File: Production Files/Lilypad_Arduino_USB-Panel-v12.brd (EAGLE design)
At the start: 125.7 x 125.7 mm, 187 parts, among them U1 MCP73831, U10 ATMEGA32U41:1, U11 MCP73831, U12 MIC5219, U2 MIC5219, U3 ATMEGA32U41:1, U4 ATMEGA32U41:1, U5 MCP73831, U6 MIC5219, U7 ATMEGA32U41:1, U8 MCP73831, U9 MIC5219, Y1 8MHz, Y2 8MHz, Y3 8MHz, Y4 8MHz

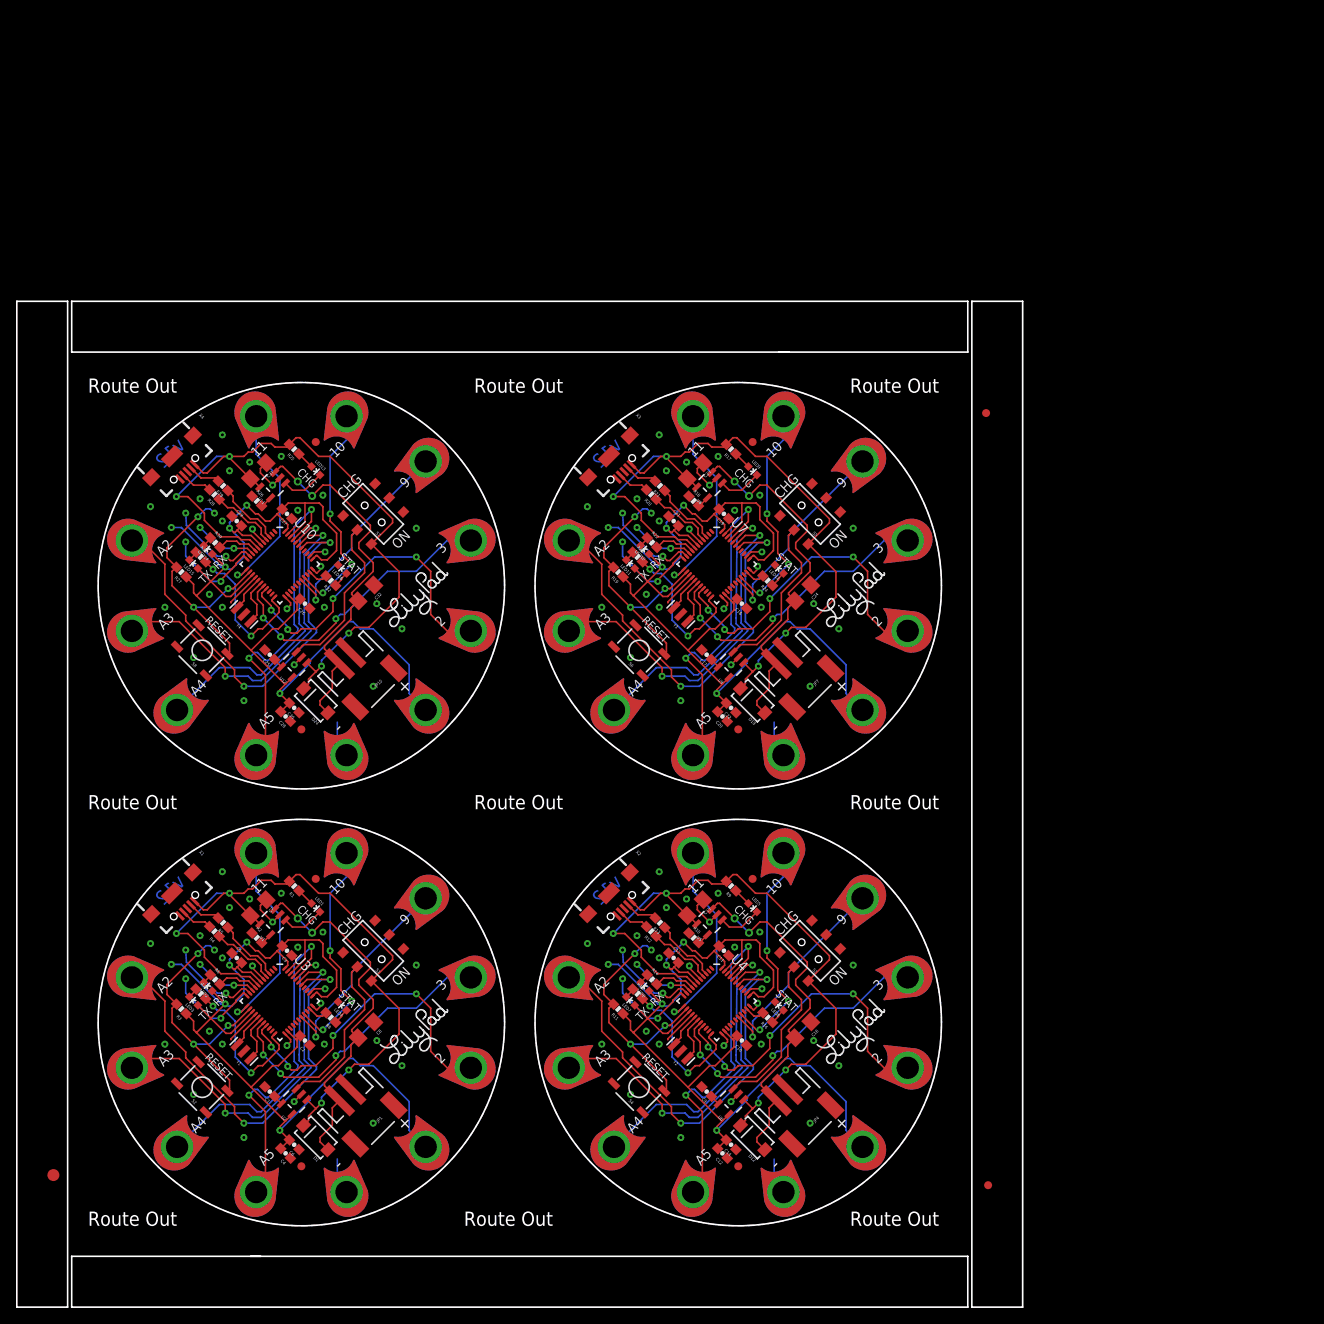
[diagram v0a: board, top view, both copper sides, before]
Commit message: created panel v12
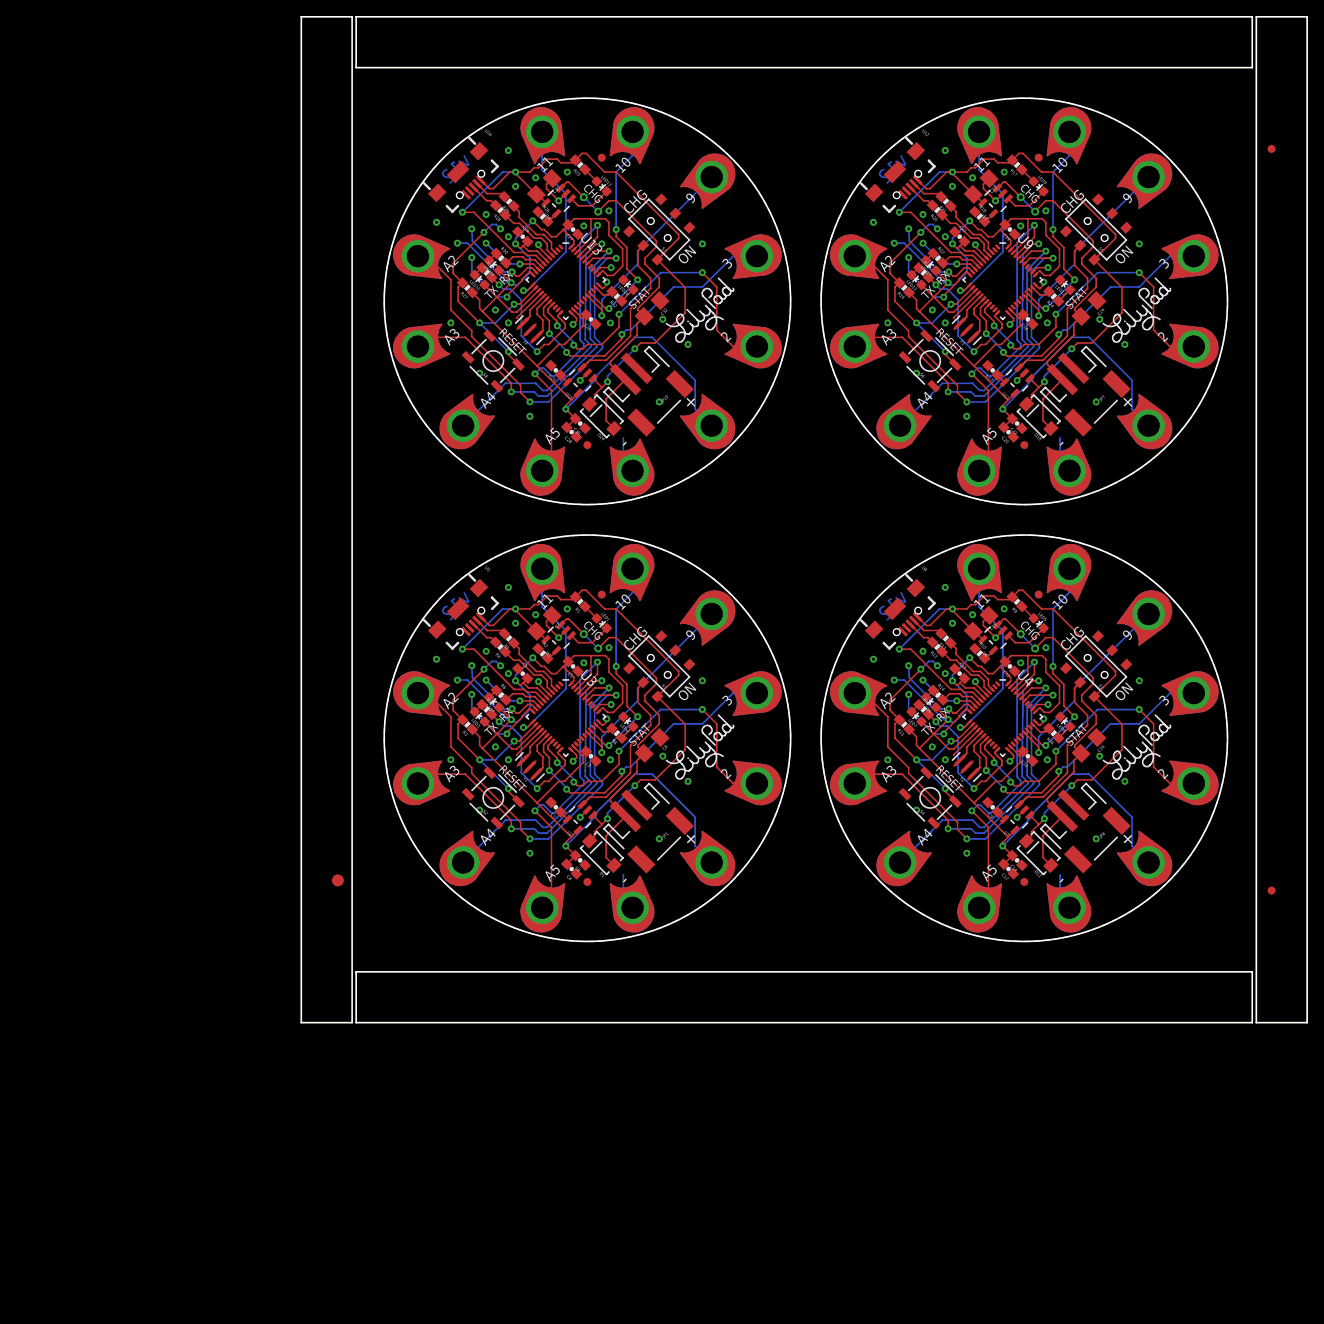
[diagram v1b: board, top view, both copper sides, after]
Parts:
- removed E$4: (no value), SparkFun-Aesthetics:FIDUCIAL-1X2
- removed X1, X2, X3, X4: (no value), Testing:USB-AB-MICRO-SMD_V03
- added E$3: (no value), SparkFun-Aesthetics:FIDUCIAL-1X2
- added U13: ATMEGA32U41:1-LESS_PASTE, Testing:QFN-44-NOPAD_1:1-LESS_PASTE
- added U14: MCP73831, SparkFun-PowerIC:SOT23-5
- added U15: MIC5219, SparkFun-PowerIC:SOT23-5
- added U16: (no value), SparkFun-Connectors:USB-AB-MICRO-SMD_V03
- E$1: device SparkFun-Aesthetics:FIDUCIAL-1.5X3 -> SparkFun-Retired:FIDUCIAL-1.5X3
- S1, S3, S5, S7: value SWITCH-DPDTSMD -> (none)
- U$11, U$16, U$6, U$7: device SparkFun-Aesthetics:SFE-LOGO-FLAME -> SparkFun-Aesthetics:SFE_LOGO_FLAME_.2
- U10: value ATMEGA32U41:1 -> MCP73831; device Testing:QFN-44-NOPAD_1:1 -> SparkFun-PowerIC:SOT23-5
- U11: value MCP73831 -> MIC5219
- U12: value MIC5219 -> (none); device SparkFun-PowerIC:SOT23-5 -> SparkFun-Connectors:USB-AB-MICRO-SMD_V03
- U3, U4: value ATMEGA32U41:1 -> ATMEGA32U41:1-LESS_PASTE; device Testing:QFN-44-NOPAD_1:1 -> Testing:QFN-44-NOPAD_1:1-LESS_PASTE
- U5, U8: value MCP73831 -> (none); device SparkFun-PowerIC:SOT23-5 -> SparkFun-Connectors:USB-AB-MICRO-SMD_V03
- U6: value MIC5219 -> MCP73831
- U7: value ATMEGA32U41:1 -> MIC5219; device Testing:QFN-44-NOPAD_1:1 -> SparkFun-PowerIC:SOT23-5
- U9: value MIC5219 -> ATMEGA32U41:1-LESS_PASTE; device SparkFun-PowerIC:SOT23-5 -> Testing:QFN-44-NOPAD_1:1-LESS_PASTE
- moved U$6 101.4 mm to (92.5, 40.6)
- moved U10 100.3 mm to (86.8, 102.7), turned to 135 degrees
- moved U12 97.1 mm to (74.2, 106.3), turned to 315 degrees
- moved U11 94.0 mm to (89.5, 80.3)
- moved U6 66.8 mm to (86.8, 48.1)
- moved U9 58.9 mm to (87.7, 92.9), turned to 315 degrees
- moved U$16 54.7 mm to (37.9, 95.2)
- moved U$11 54.7 mm to (92.5, 95.2)
- moved S2 51.3 mm to (24.0, 28.1)
- moved S4 51.3 mm to (78.6, 28.1)
- moved S6 51.3 mm to (78.6, 82.7)
- moved S8 51.3 mm to (24.0, 82.7)
- moved E$1 51.2 mm to (4.57, 17.8)
- moved JP11 50.4 mm to (35.8, 72.2)
- moved R19 50.4 mm to (75.4, 91.9)
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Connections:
- removed net N$23 (its old number): S3.2, U6.3
- removed net N$27 (its old number): C9.1, U6.4
- removed net N$36 (its old number): R12.2, X2.ID1
- removed net N$44 (its old number): X2.D+1
- removed net N$57 (its old number): R21.2, X3.D-1
- removed net N$58 (its old number): R20.2, X3.ID1
- removed net N$63 (its old number): D13.1, U7.19
- removed net N$78 (its old number): A13.1, U10.38
- removed net N$79 (its old number): R29.2, X4.D-1
- removed net N$84 (its old number): U10.16, Y4.3
- removed net N$85: D19.1, U10.19
- removed net N$86: D21.1, U10.18
- removed net N$88: X4.D+1
- new net N$24: LED5.C, U6.1
- new net N$34: R13.2, U8.D-1
- new net N$43: S5.2, U11.3
- new net N$46: R18.2, U10.5
- new net N$59: U9.17, Y3.1
- new net N$60: U9.16, Y3.3
- new net N$68: C25.1, U15.4
- new net N$81: U13.16, Y4.3
- new net N$82: D19.1, U13.19
- net 3.3V1: now also U7.5; no longer U6.5
- net 3.3V2: now also U11.5, U9.14, U9.24, U9.34, U9.42, U9.44, U9.6; no longer U7.14, U7.24, U7.34, U7.42, U7.44, U7.6, U9.5
- net 3.3V3: now also U13.14, U13.24, U13.34, U13.42, U13.44, U13.6, U15.5; no longer U10.14, U10.24, U10.34, U10.42, U10.44, U10.6, U12.5
- net 5V: now also U5.VBUS1; no longer X1.VBUS1
- net 5V1: now also U6.4, U7.1, U8.VBUS1; no longer U5.4, U6.1, X2.VBUS1
- net 5V2: now also U10.4, U11.1, U12.VBUS1, U9.7; no longer U7.7, U8.4, U9.1, X3.VBUS1
- net 5V3: now also U13.7, U14.4, U15.1, U16.VBUS1; no longer U10.7, U11.4, U12.1, X4.VBUS1
- net D+2: now also U9.4; no longer U7.4
- net D+3: now also U13.4; no longer U10.4
- net D-2: now also U9.3; no longer U7.3
- net D-3: now also U13.3; no longer U10.3
- net GND: now also U5.GND1; no longer X1.GND1
- net GND1: now also U7.2, U8.GND1; no longer U5.2, X2.GND1
- net GND2: now also U10.2, U11.2, U12.GND1, U9.15, U9.23, U9.33, U9.35, U9.43, U9.5; no longer U7.15, U7.23, U7.33, U7.35, U7.43, U7.5, U8.2, U9.2, X3.GND1
- net GND3: now also U13.15, U13.23, U13.33, U13.35, U13.43, U13.5, U14.2, U15.2, U16.GND1; no longer U10.15, U10.23, U10.33, U10.35, U10.43, U10.5, U11.2, U12.2, X4.GND1
- net MISO2: now also U9.11; no longer U7.11
- net MISO3: now also U13.11; no longer U10.11
- net MOSI2: now also U9.10; no longer U7.10
- net MOSI3: now also U13.10; no longer U10.10
- net N$19: now also U5.D-1; no longer X1.D-1
- net N$20: now also U5.D+1; no longer X1.ID1
- net N$22: now also S3.2, U7.3; no longer X1.D+1
- net N$25: now also R10.2, U6.5; no longer LED5.C, U5.1
- net N$26: now also C9.1, U7.4; no longer R10.2, U5.5
- net N$35: now also R12.2, U8.D+1; no longer R13.2, X2.D-1
- net N$45: now also LED9.C, U10.1; no longer S5.2, U9.3
- net N$47: now also C17.1, U11.4; no longer LED9.C, U8.1
- net N$48: now also D17.1, U9.12; no longer R18.2, U8.5
- net N$49: now also D16.1, U9.30; no longer C17.1, U9.4
- net N$50: now also D14.1, U9.29; no longer D17.1, U7.12
- net N$51: now also A11.1, U9.41; no longer D16.1, U7.30
- net N$52: now also A12.1, U9.40; no longer D14.1, U7.29
- net N$53: now also A10.1, U9.39; no longer A11.1, U7.41
- net N$54: now also A9.1, U9.38; no longer A12.1, U7.40
- net N$55: now also R21.2, U12.D-1; no longer A10.1, U7.39
- net N$56: now also R20.2, U12.D+1; no longer A9.1, U7.38
- net N$61: now also D13.1, U9.19; no longer U7.17, Y3.1
- net N$62: now also D15.1, U9.18; no longer U7.16, Y3.3
- net N$64: now also S7.2, U15.3; no longer D15.1, U7.18
- net N$66: now also LED13.C, U14.1; no longer X3.D+1
- net N$67: now also R26.2, U14.5; no longer S7.2, U12.3
- net N$69: now also D23.1, U13.12; no longer LED13.C, U11.1
- net N$70: now also D22.1, U13.30; no longer R26.2, U11.5
- net N$71: now also D20.1, U13.29; no longer C25.1, U12.4
- net N$72: now also A15.1, U13.41; no longer D23.1, U10.12
- net N$73: now also A16.1, U13.40; no longer D22.1, U10.30
- net N$74: now also A14.1, U13.39; no longer D20.1, U10.29
- net N$75: now also A13.1, U13.38; no longer A15.1, U10.41
- net N$76: now also R29.2, U16.D-1; no longer A16.1, U10.40
- net N$77: now also R28.2, U16.D+1; no longer A14.1, U10.39
- net N$80: now also U13.17, Y4.1; no longer R28.2, X4.ID1
- net N$83: now also D21.1, U13.18; no longer U10.17, Y4.1
- net RESET2: now also U9.13; no longer U7.13
- net RESET3: now also U13.13; no longer U10.13
- net RX_LED2: now also U9.8; no longer U7.8
- net RX_LED3: now also U13.8; no longer U10.8
- net SCK2: now also U9.9; no longer U7.9
- net SCK3: now also U13.9; no longer U10.9
- net TX_LED2: now also U9.22; no longer U7.22
- net TX_LED3: now also U13.22; no longer U10.22
- net USER_LED2: now also U9.32; no longer U7.32
- net USER_LED3: now also U13.32; no longer U10.32
- net V_BATT1: now also U6.3; no longer U5.3
- net V_BATT2: now also U10.3; no longer U8.3
- net V_BATT3: now also U14.3; no longer U11.3
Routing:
- net N$78 (its old number): track 53.9 -> 0.00 mm, vias 2 -> 0
- net N$56: track 53.9 -> 3.72 mm, vias 2 -> 0
- net N$77: track 45.9 -> 3.72 mm, vias 2 -> 0
- net N$55: track 45.9 -> 4.08 mm, vias 2 -> 0
- net N$85: track 41.6 -> 0.00 mm, vias 4 -> 0
- net N$63 (its old number): track 41.6 -> 0.00 mm, vias 4 -> 0
- net N$82: track 0.00 -> 41.6 mm, vias 0 -> 4
- net N$86: track 37.3 -> 0.00 mm, vias 3 -> 0
- net N$61: track 5.90 -> 41.6 mm, vias 0 -> 4
- net N$76: track 38.4 -> 4.08 mm, vias 1 -> 0
- net N$62: track 4.52 -> 37.3 mm, vias 0 -> 3
- net N$83: track 5.90 -> 37.3 mm, vias 0 -> 3
- net N$70: track 1.54 -> 28.7 mm, vias 0 -> 3
- net N$49: track 2.71 -> 28.7 mm, vias 0 -> 3
- net N$71: track 2.71 -> 26.2 mm, vias 0 -> 1
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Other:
- outline, holes or cut-outs redrawn
- board text removed: "Route Out"
